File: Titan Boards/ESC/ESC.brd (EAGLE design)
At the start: 101.6 x 101.6 mm, 105 parts, among them IC1 7425D, IC2 74AHC1G08DBV, Q1 5.8A/30V/35mΩ, Q2 5.8A/30V/35mΩ, Q3 5.8A/30V/35mΩ, Q4 5.8A/30V/35mΩ, Q5 5.8A/30V/35mΩ, Q6 5.8A/30V/35mΩ, Q7 5.8A/30V/35mΩ, Q8 5.8A/30V/35mΩ

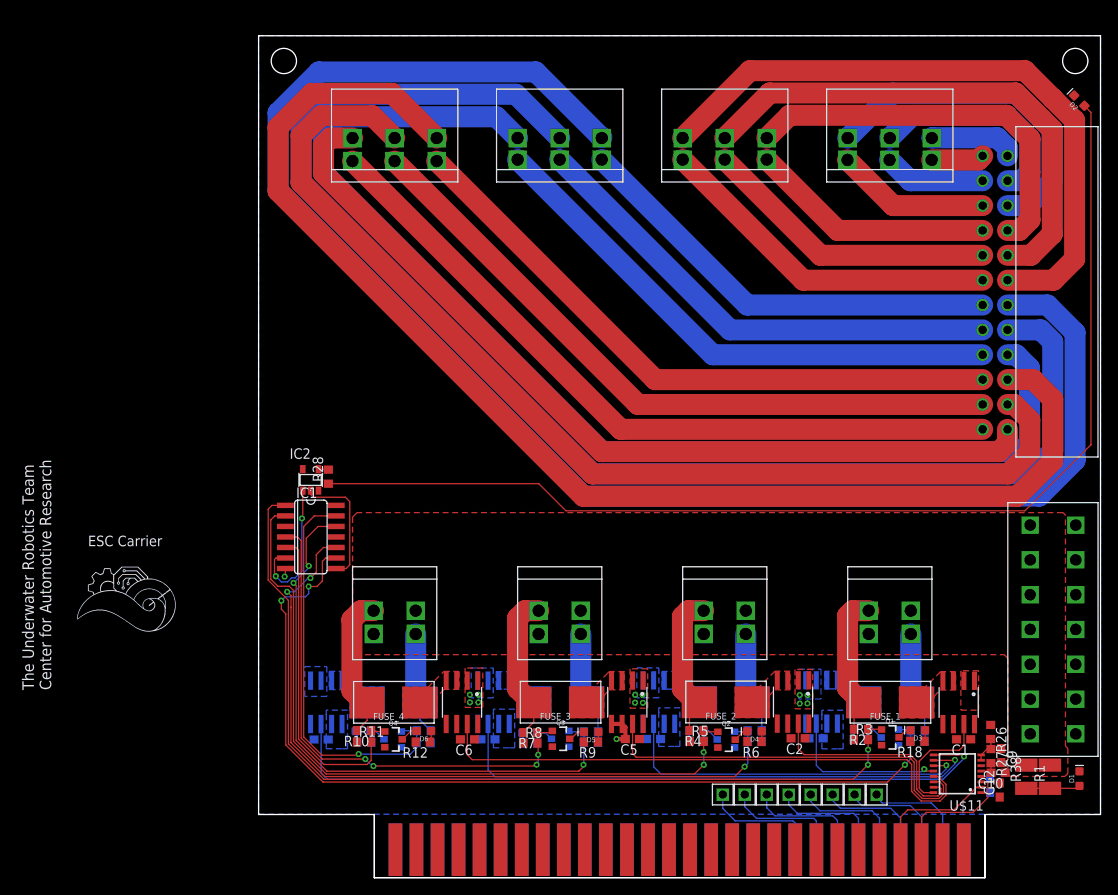
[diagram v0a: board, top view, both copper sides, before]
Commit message: FInal ESC after review
See summary
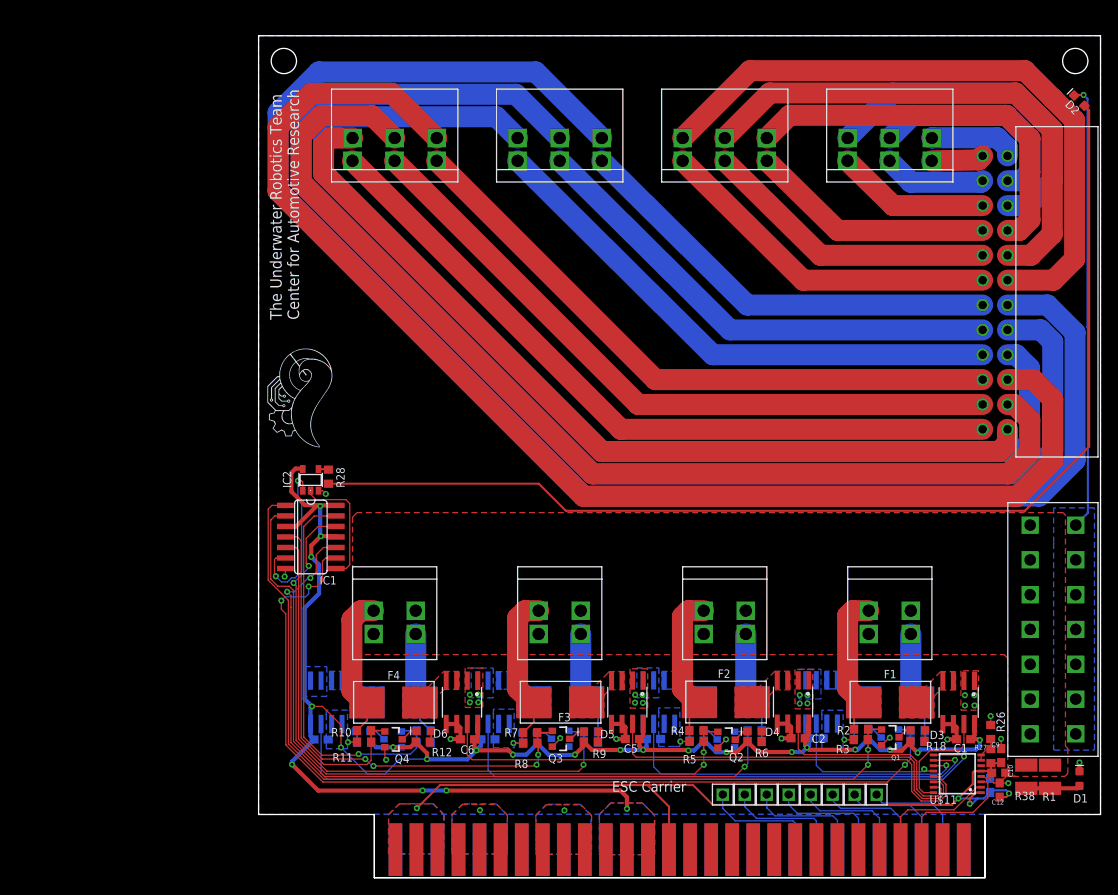
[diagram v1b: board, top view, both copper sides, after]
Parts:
- moved 3-PIN_6 0.15 mm to (56.3, 86.5)
- moved 3-PIN_7 0.15 mm to (36.3, 86.5)
- moved 3-PIN_5 0.11 mm to (76.1, 86.5)
- moved C10 0.07 mm to (89.3, 12.7)
- renumbered FUSE_1 to F1, FUSE_2 to F2, FUSE_3 to F3, FUSE_4 to F4, FUSE_5 to F5, FUSE_6 to F6, FUSE_7 to F7, FUSE_8 to F8
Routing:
- net +5V: track 0.00 -> 222.5 mm, vias 0 -> 24
- net +3V3: track 3.71 -> 97.0 mm, vias 0 -> 4
- net GND: track 5.34 -> 92.4 mm, vias 14 -> 37
- net NOR_1_OUT: track 17.2 -> 20.2 mm
- added copper zone on layer 1, net +3V3
- added copper zone on layer 16, net +3V3
- added copper zone on layer 1, net +5V
- added copper zone on layer 16, net +5V
